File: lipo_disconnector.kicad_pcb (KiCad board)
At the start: 2 copper layers, 35 x 21.3 mm, 16 parts, among them J1 Conn_Batt1, J2 Conn_Batt2, J3 Conn_Jumper, P1 Conn_01x01_Male, P2 Conn_01x01_Male

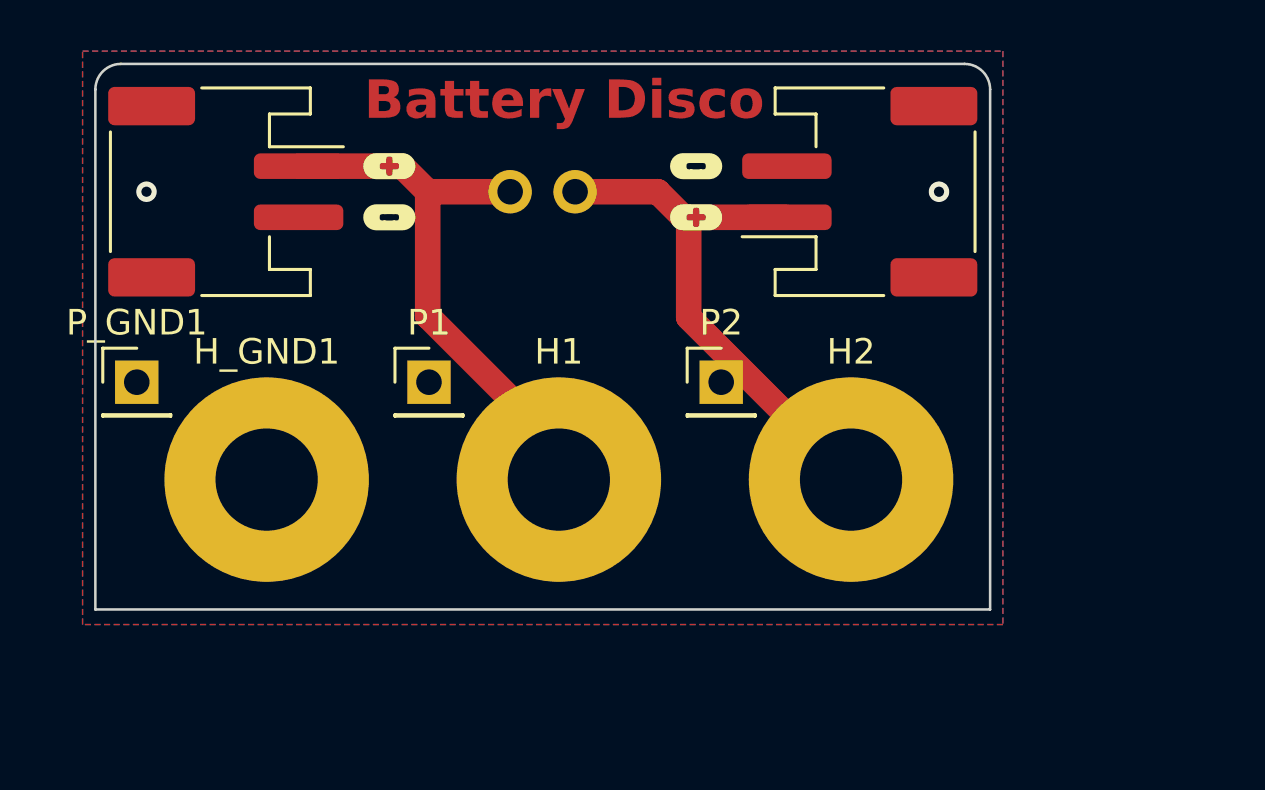
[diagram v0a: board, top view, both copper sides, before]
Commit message: Design updated
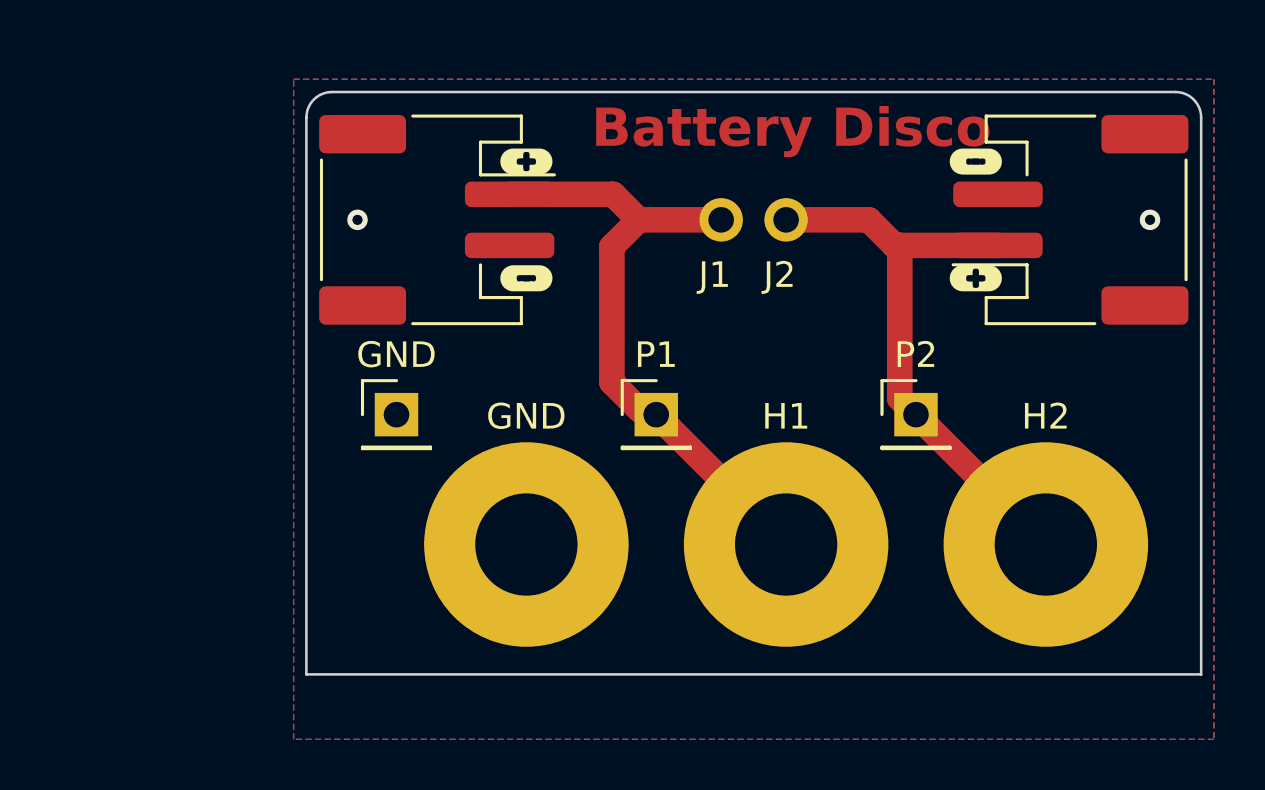
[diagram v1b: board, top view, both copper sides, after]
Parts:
- removed H_GND1: MountingHole_Pad, MountingHole:MountingHole_4mm_Pad
- added GND: MountingHole_Pad, MountingHole:MountingHole_4mm_Pad, F.Cu at (149.9, 114.3)
- moved kibuzzard-62E1C2B7 11.2 mm to (167.4, 103.9)
- moved kibuzzard-62E1C2B7 10.9 mm to (167.4, 99.3)
- moved GND 10.2 mm to (144.8, 109.2)
- moved H1 9.25 mm to (160.0, 114.3)
- moved P1 8.98 mm to (154.9, 109.2)
- moved J1 8.33 mm to (146.4, 101.6)
- moved J2 8.33 mm to (171.2, 101.6)
- moved J3 8.33 mm to (157.5, 101.6)
- moved kibuzzard-62E2BF27 8.04 mm to (158.5, 97.9)
- moved kibuzzard-62E2BF3F 8.04 mm to (158.5, 99.6)
- moved kibuzzard-62E2BF4D 8.04 mm to (158.5, 103.4)
- moved H2 8.03 mm to (170.2, 114.3)
- moved P2 7.73 mm to (165.1, 109.2)
- moved kibuzzard-62E1C2B7 5.87 mm to (149.9, 103.9)
- moved kibuzzard-62E1C2B7 5.36 mm to (149.9, 99.3)
- renumbered P_GND1 to GND
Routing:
- net Net-(J1-Pin_1): track 22.1 -> 23.7 mm
- net Net-(J2-Pin_1): track 21.6 -> 22.8 mm
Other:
- board size 35 x 21.3 mm -> 35 x 22.8 mm
- board text added: "J1"
- board text added: "J2"

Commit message: Update lipo_disconnector.kicad_pcb
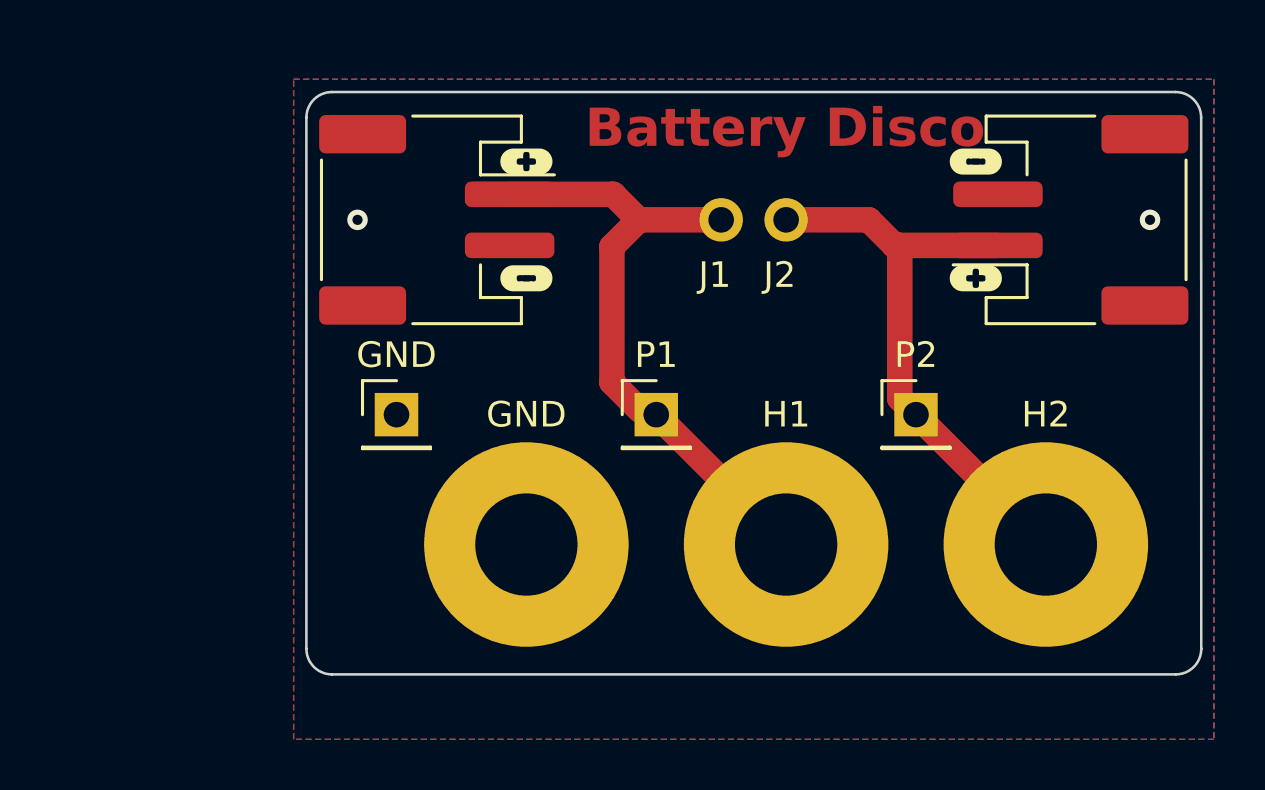
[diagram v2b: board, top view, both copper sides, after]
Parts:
- removed kibuzzard-62E2BF27: G***, kibuzzard-62E2BF27
- removed kibuzzard-62E2BF3F: G***, kibuzzard-62E2BF3F
- removed kibuzzard-62E2BF4D: G***, kibuzzard-62E2BF4D
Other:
- outline, holes or cut-outs redrawn
- board text added: "Always check polarity. Don't cross the streams."
- board text added: "https://opendeved.net/battdisco"
